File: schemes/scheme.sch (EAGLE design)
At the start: 1 part

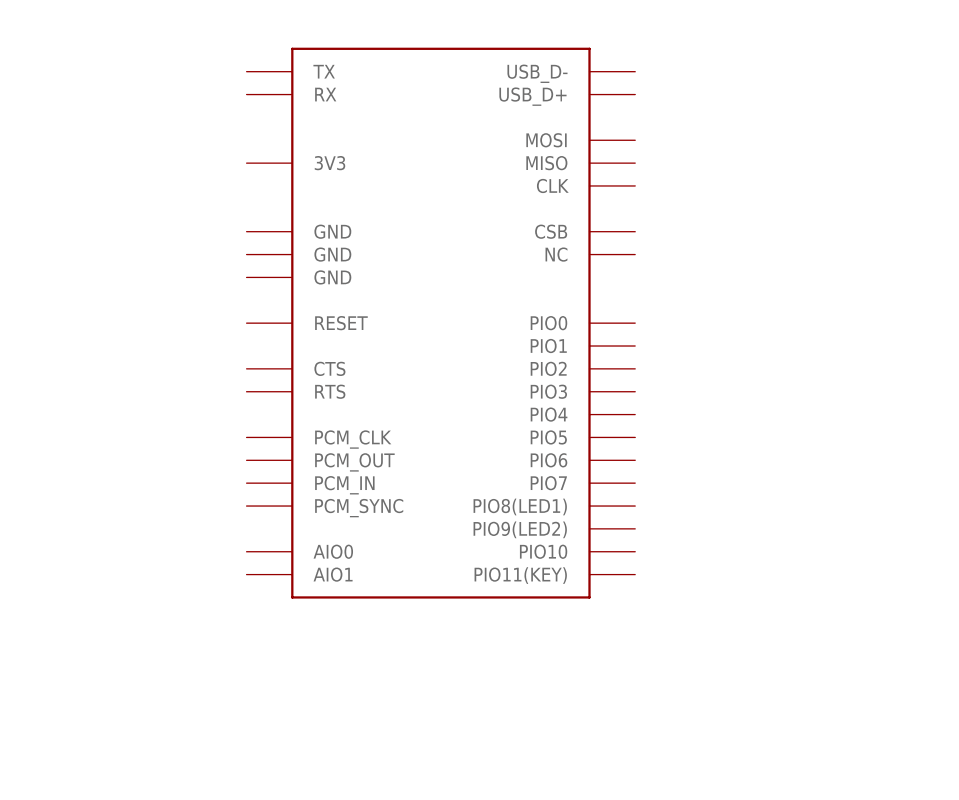
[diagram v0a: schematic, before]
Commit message: Scheme done
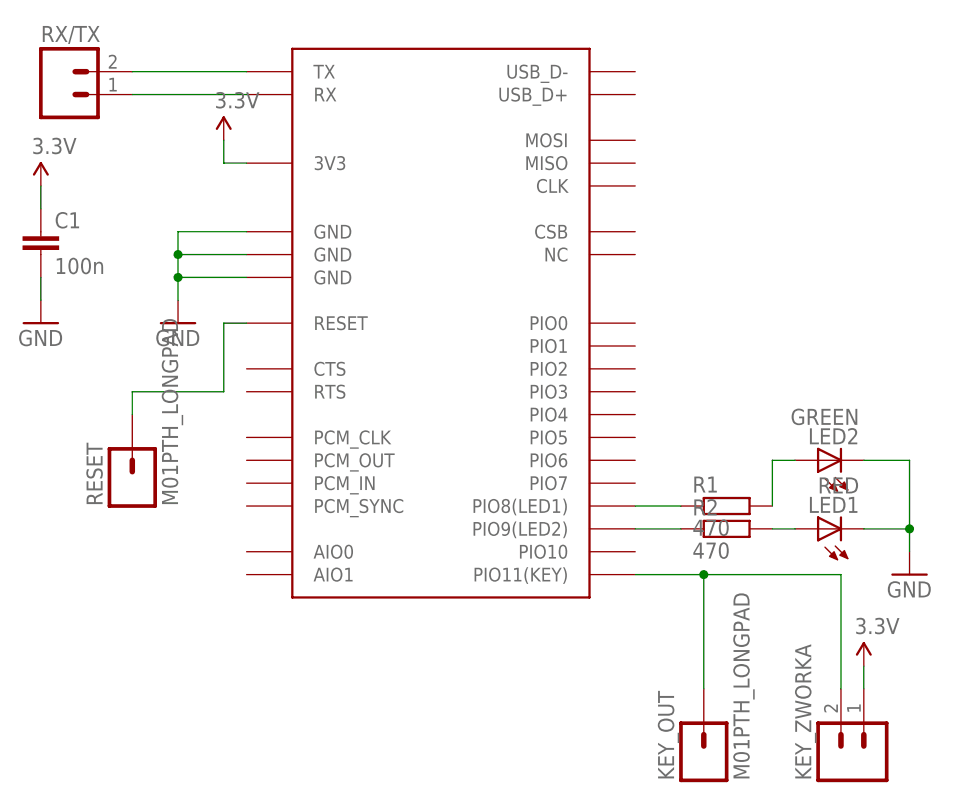
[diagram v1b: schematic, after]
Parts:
- added C1: 100n, rcl:C-EUC0805
- added KEY_OUT, RESET: M01PTH_LONGPAD, SparkFun:M01PTH_LONGPAD
- added KEY_ZWORKA, RX/TX: (no value), SparkFun:M02
- added LED1: RED, SparkFun:LED0603
- added LED2: GREEN, SparkFun:LED0603
- added R1, R2: 470, rcl:R-EU_R0805
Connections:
- new net 3.3V: C1.1, IC1.3V3, KEY_ZWORKA.1
- new net GND: C1.2, IC1.GND@1, IC1.GND@2, IC1.GND@3, LED1.C, LED2.C
- new net N$1: IC1.PIO11(KEY), KEY_OUT.1, KEY_ZWORKA.2
- new net N$2: IC1.PIO8(LED1), R1.1
- new net N$3: IC1.PIO9(LED2), R2.1
- new net N$4: LED2.A, R1.2
- new net N$5: LED1.A, R2.2
- new net N$6: IC1.RESET, RESET.1
- new net N$7: IC1.TX, RX/TX.2
- new net N$8: IC1.RX, RX/TX.1
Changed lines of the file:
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@@
 <layer number="48" name="Document" color="7" fill="1" visible="no" active="no"/>
 <layer number="49" name="Reference" color="7" fill="1" visible="no" active="no"/>
+<layer number="50" name="dxf" color="7" fill="1" visible="no" active="no"/>
 <layer number="51" name="tDocu" color="7" fill="1" visible="no" active="no"/>
 <layer number="52" name="bDocu" color="7" fill="1" visible="no" active="no"/>
+<layer number="53" name="tGND_GNDA" color="7" fill="9" visible="no" active="no"/>
+<layer number="54" name="bGND_GNDA" color="1" fill="9" visible="no" active="no"/>
+<layer number="56" name="wert" color="7" fill="1" visible="no" active="no"/>
 <layer number="91" name="Nets" color="2" fill="1" visible="yes" active="yes"/>
 <layer number="92" name="Busses" color="1" fill="1" visible="yes" active="yes"/>
@@
 <layer number="97" name="Info" color="7" fill="1" visible="yes" active="yes"/>
 <layer number="98" name="Guide" color="6" fill="1" visible="yes" active="yes"/>
+<layer number="100" name="Muster" color="7" fill="1" visible="no" active="no"/>
+<layer number="101" name="Patch_Top" color="12" fill="4" visible="yes" active="yes"/>
+<layer number="102" name="Vscore" color="7" fill="1" visible="yes" active="yes"/>
+<layer number="103" name="tMap" color="7" fill="1" visible="yes" active="yes"/>
+<layer number="104" name="Name" color="16" fill="1" visible="yes" active="yes"/>
+<layer number="105" name="tPlate" color="7" fill="1" visible="yes" active="yes"/>
+<layer number="106" name="bPlate" color="7" fill="1" visible="yes" active="yes"/>
+<layer number="107" name="Crop" color="7" fill="1" visible="yes" active="yes"/>
+<layer number="116" name="Patch_BOT" color="9" fill="4" visible="yes" active="yes"/>
+<layer number="121" name="_tsilk" color="7" fill="1" visible="yes" active="yes"/>
+<layer number="122" name="_bsilk" color="7" fill="1" visible="yes" active="yes"/>
+<layer number="151" name="HeatSink" color="7" fill="1" visible="yes" active="yes"/>
+<layer number="200" name="200bmp" color="1" fill="10" visible="yes" active="yes"/>
+<layer number="201" name="201bmp" color="2" fill="10" visible="yes" active="yes"/>
+<layer number="202" name="202bmp" color="3" fill="10" visible="yes" active="yes"/>
+<layer number="203" name="203bmp" color="4" fill="10" visible="yes" active="yes"/>
+<layer number="204" name="204bmp" color="5" fill="10" visible="yes" active="yes"/>
+<layer number="205" name="205bmp" color="6" fill="10" visible="yes" active="yes"/>
+<layer number="206" name="206bmp" color="7" fill="10" visible="yes" active="yes"/>
+<layer number="207" name="207bmp" color="8" fill="10" visible="yes" active="yes"/>
+<layer number="208" name="208bmp" color="9" fill="10" visible="yes" active="yes"/>
+<layer number="250" name="Descript" color="3" fill="1" visible="no" active="no"/>
+<layer number="251" name="SMDround" color="12" fill="11" visible="no" active="no"/>
+<layer number="254" name="cooling" color="7" fill="1" visible="yes" active="yes"/>
 </layers>
 <schematic xreflabel="%F%N/%S.%C%R" xrefpart="/%S.%C%R">
@@
 <parts>
 <part name="IC1" library="HC-05" deviceset="HC-05" device=""/>
+<part name="KEY_ZWORKA" library="SparkFun" deviceset="M02" device=""/>
+<part name="P+1" library="SparkFun" deviceset="3.3V" device=""/>
+<part name="KEY_OUT" library="SparkFun" deviceset="M01" device="PTH_LONGPAD"/>
+<part name="R1" library="rcl" deviceset="R-EU_" device="R0805" value="470"/>
+<part name="R2" library="rcl" deviceset="R-EU_" device="R0805" value="470"/>
+<part name="LED1" library="SparkFun" deviceset="LED" device="0603" value="RED"/>
+<part name="LED2" library="SparkFun" deviceset="LED" device="0603" value="GREEN"/>
+<part name="GND1" library="SparkFun" deviceset="GND" device=""/>
+<part name="P+2" library="SparkFun" deviceset="3.3V" device=""/>
+<part name="GND2" library="SparkFun" deviceset="GND" device=""/>
+<part name="RX/TX" library="SparkFun" deviceset="M02" device=""/>
+<part name="C1" library="rcl" deviceset="C-EU" device="C0805" value="100n"/>
+<part name="P+3" library="SparkFun" deviceset="3.3V" device=""/>
+<part name="GND3" library="SparkFun" deviceset="GND" device=""/>
+<part name="RESET" library="SparkFun" deviceset="M01" device="PTH_LONGPAD"/>
 </parts>
 <sheets>
@@
 <instances>
 <instance part="IC1" gate="G$1" x="48.26" y="40.64"/>
+<instance part="KEY_ZWORKA" gate="G$1" x="86.36" y="-10.16" rot="R90"/>
+<instance part="P+1" gate="G$1" x="86.36" y="0"/>
+<instance part="KEY_OUT" gate="G$1" x="68.58" y="-10.16" rot="R90"/>
+<instance part="R1" gate="G$1" x="71.12" y="17.78"/>
+<instance part="R2" gate="G$1" x="71.12" y="15.24"/>
+<instance part="LED1" gate="G$1" x="81.28" y="15.24" rot="R90"/>
+<instance part="LED2" gate="G$1" x="81.28" y="22.86" rot="R90"/>
+<instance part="GND1" gate="1" x="91.44" y="10.16"/>
+<instance part="P+2" gate="G$1" x="15.24" y="58.42"/>
+<instance part="GND2" gate="1" x="10.16" y="38.1"/>
+<instance part="RX/TX" gate="G$1" x="-2.54" y="63.5"/>
+<instance part="C1" gate="G$1" x="-5.08" y="48.26"/>
+<instance part="P+3" gate="G$1" x="-5.08" y="53.34"/>
+<instance part="GND3" gate="1" x="-5.08" y="38.1"/>
+<instance part="RESET" gate="G$1" x="5.08" y="20.32" rot="R90"/>
 </instances>
 <busses>
 </busses>
 <nets>
+<net name="N$1" class="0">
+<segment>
+<pinref part="IC1" gate="G$1" pin="PIO11(KEY)"/>
+<pinref part="KEY_ZWORKA" gate="G$1" pin="2"/>
+<wire x1="60.96" y1="10.16" x2="68.58" y2="10.16" width="0.1524" layer="91"/>
+<wire x1="68.58" y1="10.16" x2="83.82" y2="10.16" width="0.1524" layer="91"/>
+<wire x1="83.82" y1="10.16" x2="83.82" y2="-2.54" width="0.1524" layer="91"/>
+<pinref part="KEY_OUT" gate="G$1" pin="1"/>
+<wire x1="68.58" y1="-2.54" x2="68.58" y2="10.16" width="0.1524" layer="91"/>
+<junction x="68.58" y="10.16"/>
+</segment>
+</net>
+<net name="3.3V" class="0">
+<segment>
+<pinref part="KEY_ZWORKA" gate="G$1" pin="1"/>
+<pinref part="P+1" gate="G$1" pin="3.3V"/>
+<wire x1="86.36" y1="-2.54" x2="86.36" y2="0" width="0.1524" layer="91"/>
+</segment>
+<segment>
+<pinref part="IC1" gate="G$1" pin="3V3"/>
+<pinref part="P+2" gate="G$1" pin="3.3V"/>
+<wire x1="17.78" y1="55.88" x2="15.24" y2="55.88" width="0.1524" layer="91"/>
+<wire x1="15.24" y1="55.88" x2="15.24" y2="58.42" width="0.1524" layer="91"/>
+</segment>
+<segment>
+<pinref part="C1" gate="G$1" pin="1"/>
+<pinref part="P+3" gate="G$1" pin="3.3V"/>
+<wire x1="-5.08" y1="50.8" x2="-5.08" y2="53.34" width="0.1524" layer="91"/>
+</segment>
+</net>
+<net name="N$2" class="0">
+<segment>
+<pinref part="IC1" gate="G$1" pin="PIO8(LED1)"/>
+<wire x1="60.96" y1="17.78" x2="66.04" y2="17.78" width="0.1524" layer="91"/>
+<pinref part="R1" gate="G$1" pin="1"/>
+</segment>
+</net>
+<net name="N$3" class="0">
+<segment>
+<pinref part="IC1" gate="G$1" pin="PIO9(LED2)"/>
+<pinref part="R2" gate="G$1" pin="1"/>
+<wire x1="60.96" y1="15.24" x2="66.04" y2="15.24" width="0.1524" layer="91"/>
+</segment>
+</net>
+<net name="N$5" class="0">
+<segment>
+<pinref part="R2" gate="G$1" pin="2"/>
+<wire x1="76.2" y1="15.24" x2="78.74" y2="15.24" width="0.1524" layer="91"/>
+<pinref part="LED1" gate="G$1" pin="A"/>
+</segment>
+</net>
+<net name="N$4" class="0">
+<segment>
+<pinref part="R1" gate="G$1" pin="2"/>
+<wire x1="76.2" y1="17.78" x2="76.2" y2="22.86" width="0.1524" layer="91"/>
+<pinref part="LED2" gate="G$1" pin="A"/>
+<wire x1="76.2" y1="22.86" x2="78.74" y2="22.86" width="0.1524" layer="91"/>
+</segment>
+</net>
+<net name="GND" class="0">
+<segment>
+<pinref part="LED1" gate="G$1" pin="C"/>
+<wire x1="86.36" y1="15.24" x2="91.44" y2="15.24" width="0.1524" layer="91"/>
+<wire x1="91.44" y1="15.24" x2="91.44" y2="12.7" width="0.1524" layer="91"/>
+<pinref part="LED2" gate="G$1" pin="C"/>
+<wire x1="86.36" y1="22.86" x2="91.44" y2="22.86" width="0.1524" layer="91"/>
+<wire x1="91.44" y1="22.86" x2="91.44" y2="15.24" width="0.1524" layer="91"/>
+<junction x="91.44" y="15.24"/>
+<pinref part="GND1" gate="1" pin="GND"/>
+</segment>
+<segment>
+<pinref part="IC1" gate="G$1" pin="GND@1"/>
+<pinref part="GND2" gate="1" pin="GND"/>
+<wire x1="17.78" y1="48.26" x2="10.16" y2="48.26" width="0.1524" layer="91"/>
+<wire x1="10.16" y1="48.26" x2="10.16" y2="45.72" width="0.1524" layer="91"/>
+<pinref part="IC1" gate="G$1" pin="GND@2"/>
+<wire x1="10.16" y1="45.72" x2="10.16" y2="43.18" width="0.1524" layer="91"/>
+<wire x1="10.16" y1="43.18" x2="10.16" y2="40.64" width="0.1524" layer="91"/>
+<wire x1="17.78" y1="45.72" x2="10.16" y2="45.72" width="0.1524" layer="91"/>
+<pinref part="IC1" gate="G$1" pin="GND@3"/>
+<wire x1="17.78" y1="43.18" x2="10.16" y2="43.18" width="0.1524" layer="91"/>
+<junction x="10.16" y="43.18"/>
+<junction x="10.16" y="45.72"/>
+</segment>
+<segment>
+<pinref part="GND3" gate="1" pin="GND"/>
+<pinref part="C1" gate="G$1" pin="2"/>
+<wire x1="-5.08" y1="40.64" x2="-5.08" y2="43.18" width="0.1524" layer="91"/>
+</segment>
+</net>
+<net name="N$7" class="0">
+<segment>
+<pinref part="IC1" gate="G$1" pin="TX"/>
+<pinref part="RX/TX" gate="G$1" pin="2"/>
+<wire x1="17.78" y1="66.04" x2="5.08" y2="66.04" width="0.1524" layer="91"/>
+</segment>
+</net>
+<net name="N$8" class="0">
+<segment>
+<pinref part="IC1" gate="G$1" pin="RX"/>
+<pinref part="RX/TX" gate="G$1" pin="1"/>
+<wire x1="17.78" y1="63.5" x2="5.08" y2="63.5" width="0.1524" layer="91"/>
+</segment>
+</net>
+<net name="N$6" class="0">
+<segment>
+<pinref part="IC1" gate="G$1" pin="RESET"/>
+<wire x1="17.78" y1="38.1" x2="15.24" y2="38.1" width="0.1524" layer="91"/>
+<wire x1="15.24" y1="38.1" x2="15.24" y2="30.48" width="0.1524" layer="91"/>
+<wire x1="15.24" y1="30.48" x2="5.08" y2="30.48" width="0.1524" layer="91"/>
+<wire x1="5.08" y1="30.48" x2="5.08" y2="27.94" width="0.1524" layer="91"/>
+<pinref part="RESET" gate="G$1" pin="1"/>
+</segment>
+</net>
 </nets>
 </sheet>
